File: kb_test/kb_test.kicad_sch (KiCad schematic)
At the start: 168 parts, among them SW1 SW_Push, SW10 SW_Push, SW11 SW_Push, SW12 SW_Push, SW13 SW_Push, SW14 SW_Push, SW15 SW_Push, SW16 SW_Push, SW17 SW_Push, SW18 SW_Push, SW19 SW_Push, SW2 SW_Push, SW20 SW_Push, SW21 SW_Push, SW22 SW_Push, SW23 SW_Push, SW24 SW_Push, SW25 SW_Push, SW26 SW_Push, SW27 SW_Push, SW28 SW_Push, SW29 SW_Push, SW3 SW_Push, SW30 SW_Push, SW31 SW_Push, SW32 SW_Push, SW33 SW_Push, SW34 SW_Push, SW35 SW_Push, SW36 SW_Push, SW37 SW_Push, SW38 SW_Push, SW39 SW_Push, SW4 SW_Push, SW40 SW_Push, SW41 SW_Push, SW42 SW_Push, SW43 SW_Push, SW44 SW_Push, SW45 SW_Push, SW46 SW_Push, SW47 SW_Push, SW48 SW_Push, SW49 SW_Push, SW5 SW_Push, SW50 SW_Push, SW51 SW_Push, SW52 SW_Push, SW53 SW_Push, SW54 SW_Push, SW55 SW_Push, SW56 SW_Push, SW57 SW_Push, SW58 SW_Push, SW59 SW_Push, SW6 SW_Push, SW60 SW_Push, SW61 SW_Push, SW62 SW_Push, SW63 SW_Push, SW64 SW_Push, SW65 SW_Push, SW66 SW_Push, SW67 SW_Push, SW68 SW_Push, SW69 SW_Push, SW7 SW_Push, SW70 SW_Push, SW71 SW_Push, SW72 SW_Push, SW73 SW_Push, SW74 SW_Push, SW75 SW_Push, SW76 SW_Push, SW77 SW_Push, SW78 SW_Push, SW79 SW_Push, SW8 SW_Push, SW80 SW_Push, SW81 SW_Push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

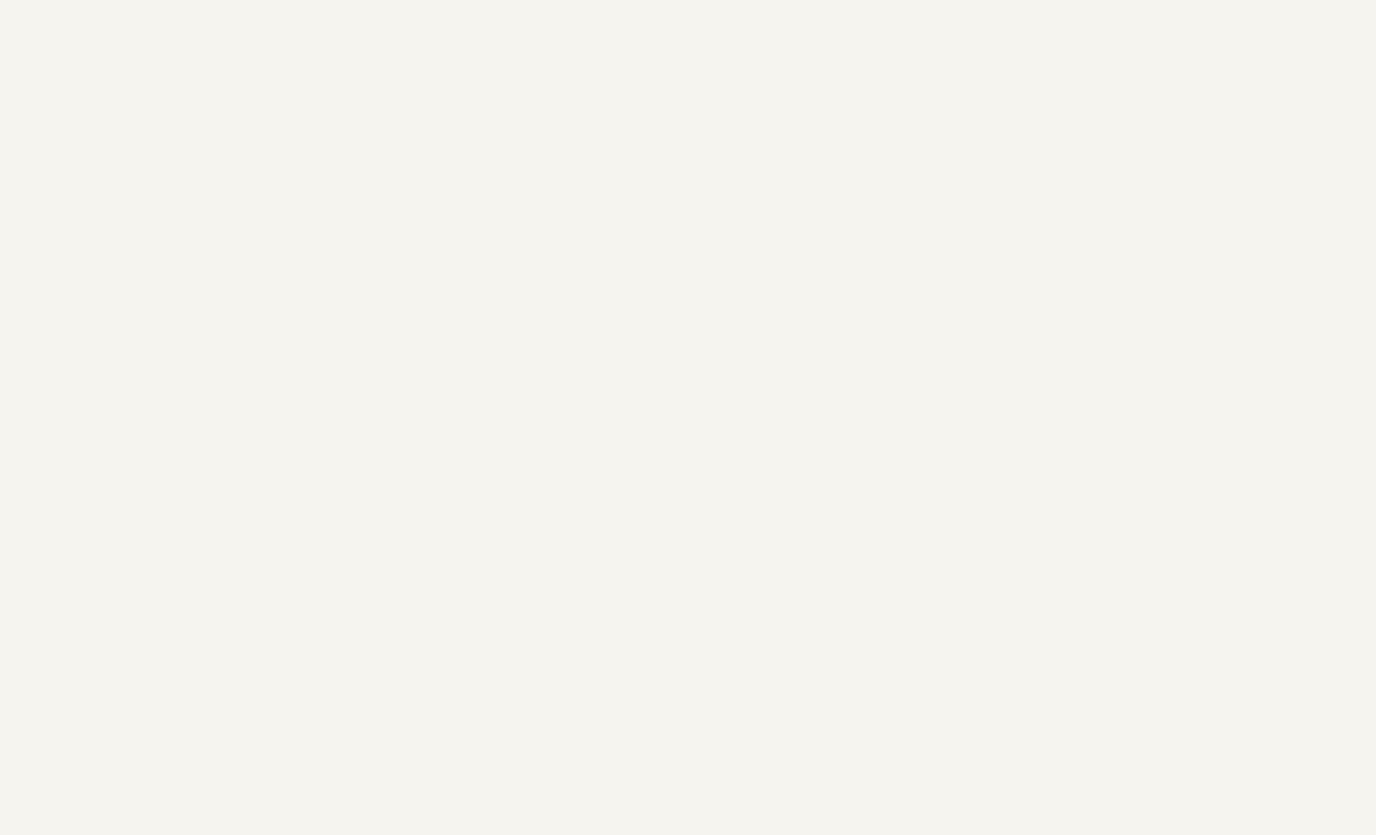
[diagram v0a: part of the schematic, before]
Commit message: Tentative placement with diodes on front
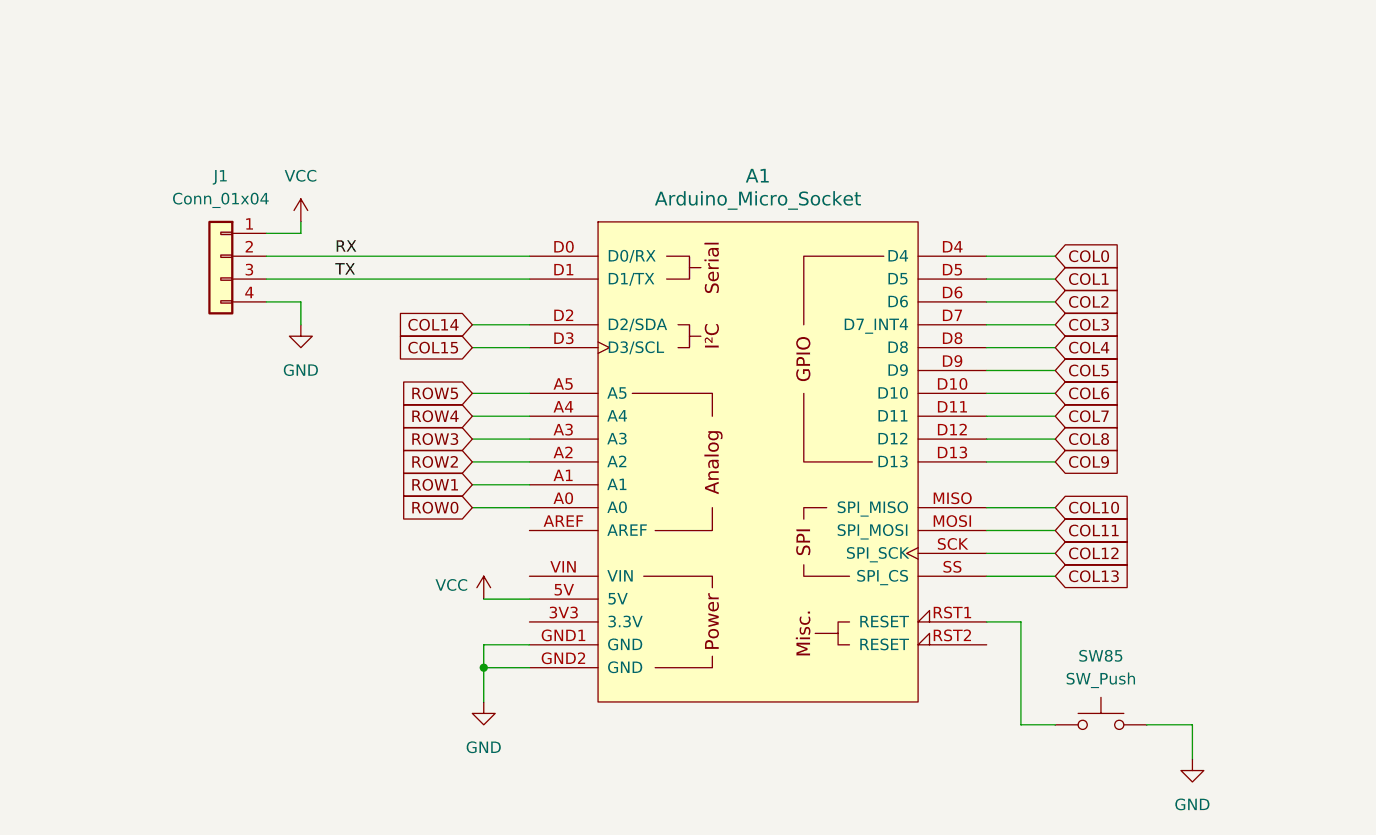
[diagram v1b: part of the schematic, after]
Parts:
- added A1: Arduino_Micro_Socket, PCM_arduino-library:Arduino_Micro_Socket, symbol arduino-kicad-library:Arduino_Micro_Socket
- added J1: Conn_01x04, Connector_PinHeader_2.54mm:PinHeader_1x04_P2.54mm_Vertical, symbol Connector_Generic:Conn_01x04
- added SW85: SW_Push, Button_Switch_THT:SW_Tactile_Straight_KSA0Axx1LFTR, symbol Switch:SW_Push
- SW1, SW10, SW11, SW12, SW13, SW14, SW15, SW16, SW17, SW18, SW19, SW2, SW20, SW21, SW22, SW23, SW24, SW25, SW26, SW27, SW28, SW29, SW3, SW30, SW31, SW32, SW33, SW34, SW35, SW36, SW37, SW38, SW39, SW4, SW40, SW41, SW42, SW43, SW44, SW45, SW46, SW47, SW48, SW49, SW5, SW50, SW51, SW52, SW53, SW54, SW55, SW56, SW57, SW58, SW59, SW6, SW60, SW61, SW62, SW63, SW64, SW65, SW66, SW67, SW68, SW69, SW7, SW70, SW71, SW72, SW73, SW74, SW75, SW76, SW77, SW78, SW79, SW8, SW80, SW81, SW82, SW83, SW84, SW9: footprint Button_Switch_Keyboard:SW_Cherry_MX_1.00u_PCB -> my_cherry:SW_Cherry_MX_1.00u_PCB
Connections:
- net COL0: now also A1.D4
- net COL1: now also A1.D5
- net COL10: now also A1.MISO (SPI_MISO)
- net COL11: now also A1.MOSI (SPI_MOSI)
- net COL12: now also A1.SCK (SPI_SCK)
- net COL13: now also A1.SS (SPI_CS)
- net COL14: now also A1.D2 (D2/SDA)
- net COL15: now also A1.D3 (D3/SCL)
- net COL2: now also A1.D6
- net COL3: now also A1.D7 (D7_INT4)
- net COL4: now also A1.D8
- net COL5: now also A1.D9
- net COL6: now also A1.D10
- net COL7: now also A1.D11
- net COL8: now also A1.D12
- net COL9: now also A1.D13
- net ROW0: now also A1.A0
- net ROW1: now also A1.A1
- net ROW2: now also A1.A2
- net ROW3: now also A1.A3
- net ROW4: now also A1.A4
- net ROW5: now also A1.A5
- new net: A1.RST1 (RESET), SW85.1
- new net GND: A1.GND1 (GND), A1.GND2 (GND), J1.4 (Pin_4), SW85.2
- new net RX: A1.D0 (D0/RX), J1.2 (Pin_2)
- new net TX: A1.D1 (D1/TX), J1.3 (Pin_3)
- new net VCC: A1.5V, J1.1 (Pin_1)
